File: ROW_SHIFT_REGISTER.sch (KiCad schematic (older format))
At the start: 27 parts, among them Q12 AO3407A, Q13 SSM3K35AMFV, Q14 SSM3K35AMFV, U10 74HC595, U11 74HC595, U12 74HC595, U9 74HC595

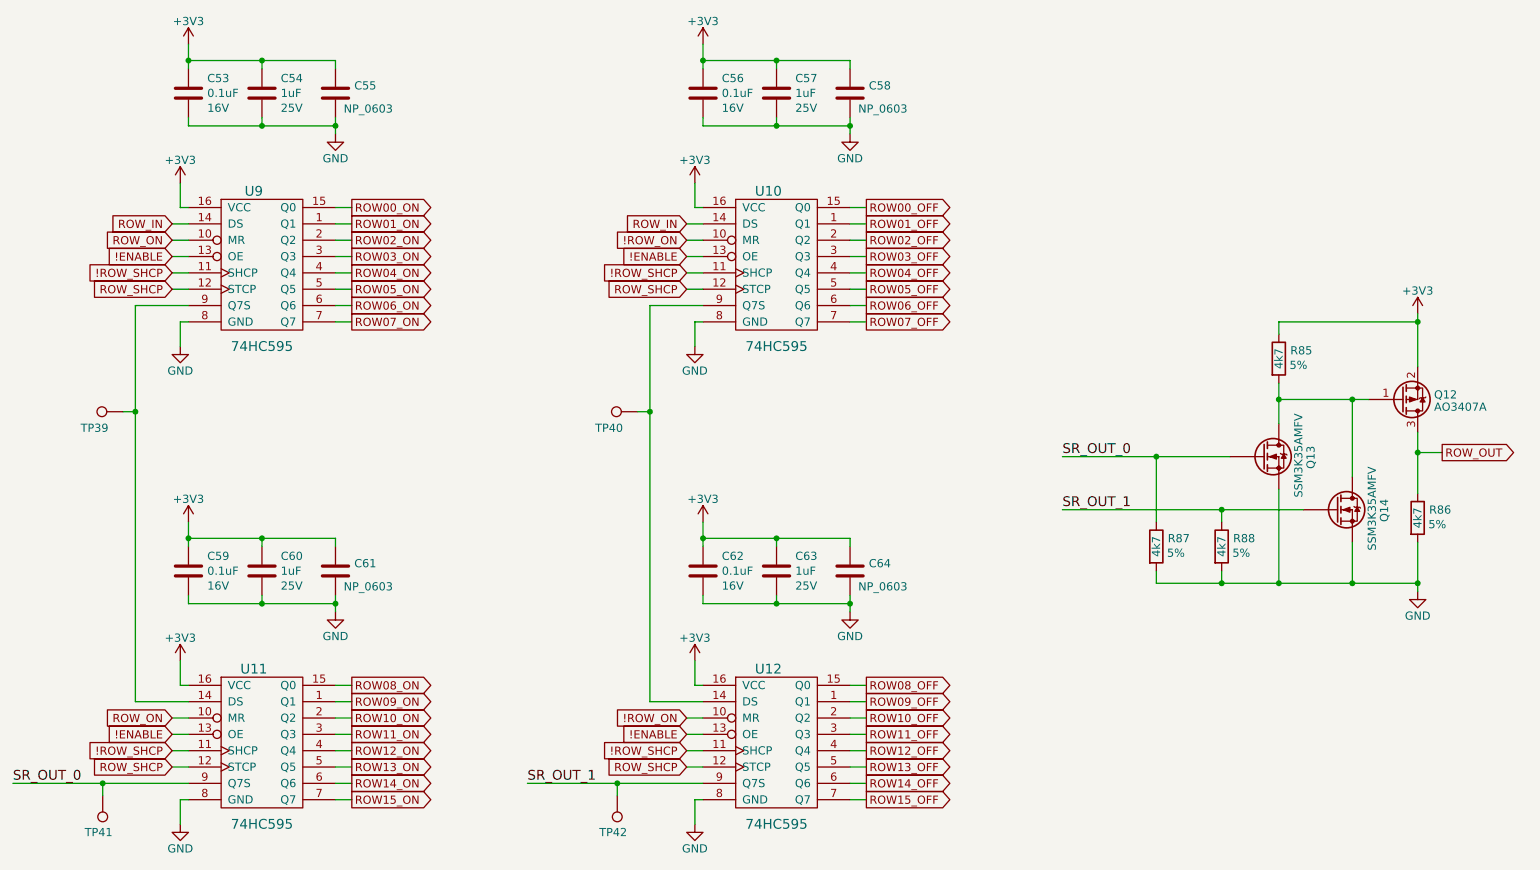
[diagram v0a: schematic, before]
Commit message: automated commit
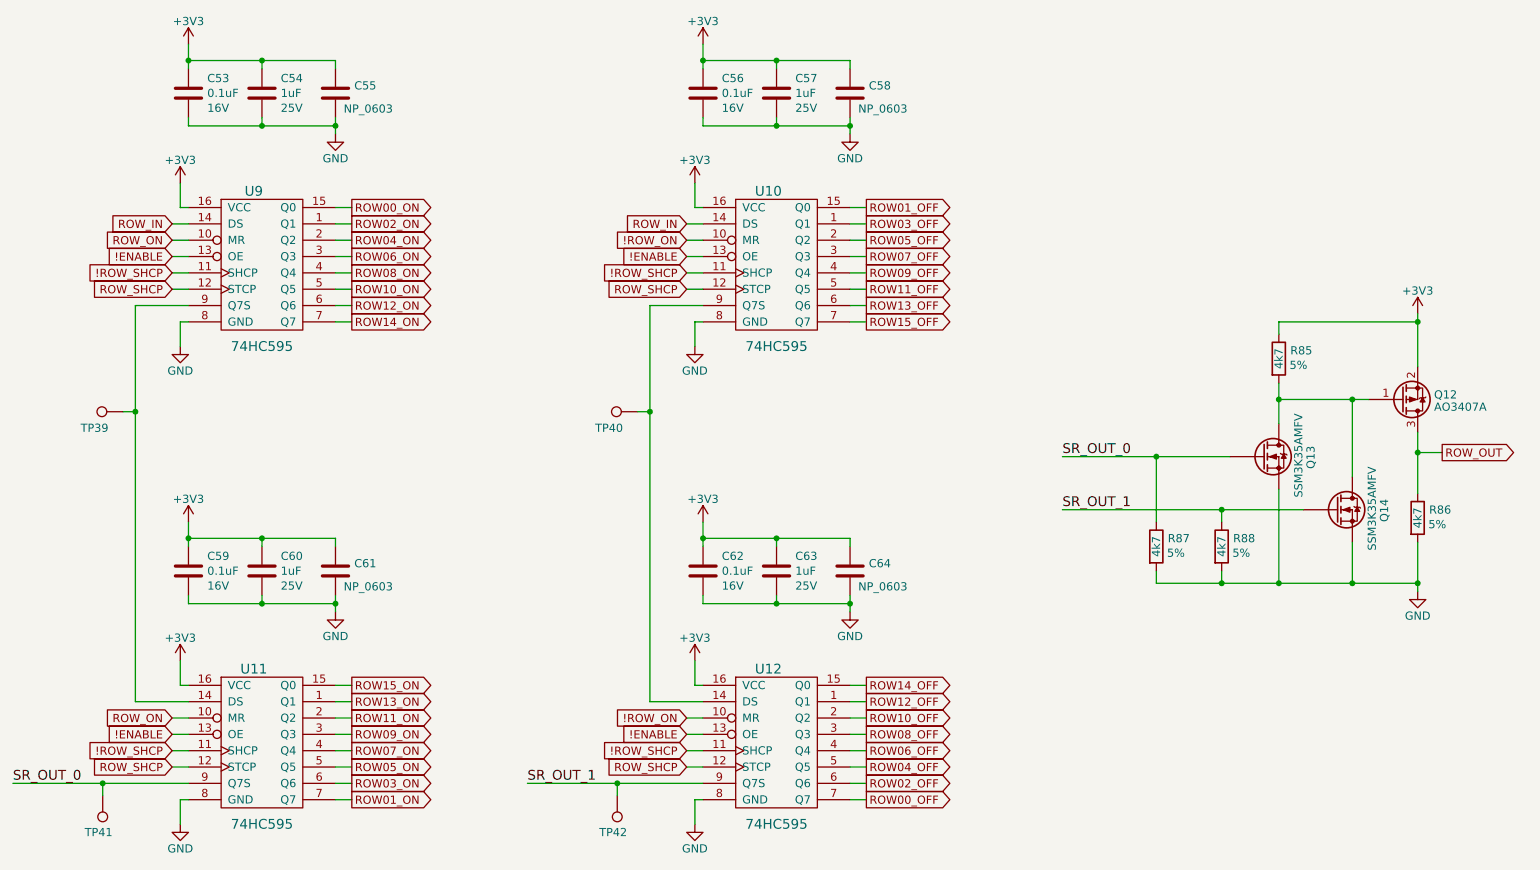
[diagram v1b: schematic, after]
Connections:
- net ROW00_OFF: now also U12.7 (Q7); no longer U10.15 (Q0)
- net ROW01_OFF: now also U10.15 (Q0); no longer U10.1 (Q1)
- net ROW01_ON: now also U11.7 (Q7); no longer U9.1 (Q1)
- net ROW02_OFF: now also U12.6 (Q6); no longer U10.2 (Q2)
- net ROW02_ON: now also U9.1 (Q1); no longer U9.2 (Q2)
- net ROW03_OFF: now also U10.1 (Q1); no longer U10.3 (Q3)
- net ROW03_ON: now also U11.6 (Q6); no longer U9.3 (Q3)
- net ROW04_OFF: now also U12.5 (Q5); no longer U10.4 (Q4)
- net ROW04_ON: now also U9.2 (Q2); no longer U9.4 (Q4)
- net ROW05_OFF: now also U10.2 (Q2); no longer U10.5 (Q5)
- net ROW05_ON: now also U11.5 (Q5); no longer U9.5 (Q5)
- net ROW06_OFF: now also U12.4 (Q4); no longer U10.6 (Q6)
- net ROW06_ON: now also U9.3 (Q3); no longer U9.6 (Q6)
- net ROW07_OFF: now also U10.3 (Q3); no longer U10.7 (Q7)
- net ROW07_ON: now also U11.4 (Q4); no longer U9.7 (Q7)
- net ROW08_OFF: now also U12.3 (Q3); no longer U12.15 (Q0)
- net ROW08_ON: now also U9.4 (Q4); no longer U11.15 (Q0)
- net ROW09_OFF: now also U10.4 (Q4); no longer U12.1 (Q1)
- net ROW09_ON: now also U11.3 (Q3); no longer U11.1 (Q1)
- net ROW10_ON: now also U9.5 (Q5); no longer U11.2 (Q2)
- net ROW11_OFF: now also U10.5 (Q5); no longer U12.3 (Q3)
- net ROW11_ON: now also U11.2 (Q2); no longer U11.3 (Q3)
- net ROW12_OFF: now also U12.1 (Q1); no longer U12.4 (Q4)
- net ROW12_ON: now also U9.6 (Q6); no longer U11.4 (Q4)
- net ROW13_OFF: now also U10.6 (Q6); no longer U12.5 (Q5)
- net ROW13_ON: now also U11.1 (Q1); no longer U11.5 (Q5)
- net ROW14_OFF: now also U12.15 (Q0); no longer U12.6 (Q6)
- net ROW14_ON: now also U9.7 (Q7); no longer U11.6 (Q6)
- net ROW15_OFF: now also U10.7 (Q7); no longer U12.7 (Q7)
- net ROW15_ON: now also U11.15 (Q0); no longer U11.7 (Q7)
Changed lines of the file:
@@
 	2925 5875 2825 5875
 Wire Wire Line
-	5975 2250 6075 2250
-Wire Wire Line
-	5975 2350 6075 2350
-Wire Wire Line
-	5975 2450 6075 2450
+	5975 5875 6075 5875
+Wire Wire Line
+	5975 5775 6075 5775
+Wire Wire Line
+	5975 5675 6075 5675
+Wire Wire Line
+	6075 5575 5975 5575
+Wire Wire Line
+	5975 5475 6075 5475
+Wire Wire Line
+	6075 5375 5975 5375
+Wire Wire Line
+	6075 5275 5975 5275
+Wire Wire Line
+	6075 5175 5975 5175
+Wire Wire Line
+	6075 2950 5975 2950
+Wire Wire Line
+	6075 2850 5975 2850
+Wire Wire Line
+	6075 2750 5975 2750
+Wire Wire Line
+	6075 2650 5975 2650
 Wire Wire Line
 	6075 2550 5975 2550
 Wire Wire Line
-	5975 2650 6075 2650
-Wire Wire Line
-	6075 2750 5975 2750
-Wire Wire Line
-	6075 2850 5975 2850
-Wire Wire Line
-	6075 2950 5975 2950
-Wire Wire Line
-	6075 5175 5975 5175
-Wire Wire Line
-	6075 5275 5975 5275
-Wire Wire Line
-	6075 5375 5975 5375
-Wire Wire Line
-	6075 5475 5975 5475
-Wire Wire Line
-	6075 5575 5975 5575
-Wire Wire Line
-	6075 5675 5975 5675
-Wire Wire Line
-	6075 5775 5975 5775
-Wire Wire Line
-	6075 5875 5975 5875
+	6075 2450 5975 2450
+Wire Wire Line
+	6075 2350 5975 2350
+Wire Wire Line
+	6075 2250 5975 2250
 $Comp
 L power:+3V3 #PWR?
@@
 Text GLabel 2925 2250 2    50   Output ~ 0
 ROW00_ON
-Text GLabel 2925 2350 2    50   Output ~ 0
-ROW01_ON
 Text GLabel 2925 2450 2    50   Output ~ 0
-ROW02_ON
+ROW04_ON
 Text GLabel 2925 2550 2    50   Output ~ 0
-ROW03_ON
+ROW06_ON
 Text GLabel 2925 2650 2    50   Output ~ 0
-ROW04_ON
+ROW08_ON
 Text GLabel 2925 2750 2    50   Output ~ 0
-ROW05_ON
+ROW10_ON
 Text GLabel 2925 2850 2    50   Output ~ 0
-ROW06_ON
+ROW12_ON
 Text GLabel 2925 2950 2    50   Output ~ 0
-ROW07_ON
-Text GLabel 2925 5175 2    50   Output ~ 0
-ROW08_ON
-Text GLabel 2925 5275 2    50   Output ~ 0
-ROW09_ON
-Text GLabel 2925 5375 2    50   Output ~ 0
-ROW10_ON
-Text GLabel 2925 5475 2    50   Output ~ 0
-ROW11_ON
-Text GLabel 2925 5575 2    50   Output ~ 0
-ROW12_ON
-Text GLabel 2925 5675 2    50   Output ~ 0
-ROW13_ON
-Text GLabel 2925 5775 2    50   Output ~ 0
 ROW14_ON
-Text GLabel 2925 5875 2    50   Output ~ 0
-ROW15_ON
-Text GLabel 6075 5175 2    50   Output ~ 0
+Text GLabel 6075 5475 2    50   Output ~ 0
 ROW08_OFF
-Text GLabel 6075 5275 2    50   Output ~ 0
+Text GLabel 6075 2650 2    50   Output ~ 0
 ROW09_OFF
 Text GLabel 6075 5375 2    50   Output ~ 0
 ROW10_OFF
-Text GLabel 6075 5475 2    50   Output ~ 0
+Text GLabel 6075 2750 2    50   Output ~ 0
 ROW11_OFF
+Text GLabel 6075 5275 2    50   Output ~ 0
+ROW12_OFF
+Text GLabel 6075 2850 2    50   Output ~ 0
+ROW13_OFF
+Text GLabel 6075 5175 2    50   Output ~ 0
+ROW14_OFF
+Text GLabel 6075 2950 2    50   Output ~ 0
+ROW15_OFF
+Text GLabel 6075 5875 2    50   Output ~ 0
+ROW00_OFF
+Text GLabel 6075 2250 2    50   Output ~ 0
+ROW01_OFF
+Text GLabel 6075 5775 2    50   Output ~ 0
+ROW02_OFF
+Text GLabel 6075 2350 2    50   Output ~ 0
+ROW03_OFF
+Text GLabel 6075 5675 2    50   Output ~ 0
+ROW04_OFF
+Text GLabel 6075 2450 2    50   Output ~ 0
+ROW05_OFF
 Text GLabel 6075 5575 2    50   Output ~ 0
-ROW12_OFF
-Text GLabel 6075 5675 2    50   Output ~ 0
-ROW13_OFF
-Text GLabel 6075 5775 2    50   Output ~ 0
-ROW14_OFF
-Text GLabel 6075 5875 2    50   Output ~ 0
-ROW15_OFF
-Text GLabel 6075 2250 2    50   Output ~ 0
-ROW00_OFF
-Text GLabel 6075 2350 2    50   Output ~ 0
-ROW01_OFF
-Text GLabel 6075 2450 2    50   Output ~ 0
-ROW02_OFF
+ROW06_OFF
 Text GLabel 6075 2550 2    50   Output ~ 0
-ROW03_OFF
-Text GLabel 6075 2650 2    50   Output ~ 0
-ROW04_OFF
-Text GLabel 6075 2750 2    50   Output ~ 0
-ROW05_OFF
-Text GLabel 6075 2850 2    50   Output ~ 0
-ROW06_OFF
-Text GLabel 6075 2950 2    50   Output ~ 0
 ROW07_OFF
 Wire Wire Line
@@
 Wire Wire Line
 	1825 2350 1925 2350
+Text GLabel 2925 5875 2    50   Output ~ 0
+ROW01_ON
+Text GLabel 2925 5775 2    50   Output ~ 0
+ROW03_ON
+Text GLabel 2925 5675 2    50   Output ~ 0
+ROW05_ON
+Text GLabel 2925 5575 2    50   Output ~ 0
+ROW07_ON
+Text GLabel 2925 5475 2    50   Output ~ 0
+ROW09_ON
+Text GLabel 2925 5375 2    50   Output ~ 0
+ROW11_ON
+Text GLabel 2925 5275 2    50   Output ~ 0
+ROW13_ON
+Text GLabel 2925 5175 2    50   Output ~ 0
+ROW15_ON
+Text GLabel 2925 2350 2    50   Output ~ 0
+ROW02_ON
 $EndSCHEMATC
